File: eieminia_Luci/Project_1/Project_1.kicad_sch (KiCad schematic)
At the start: 10 parts, among them J2 Conn_01x05

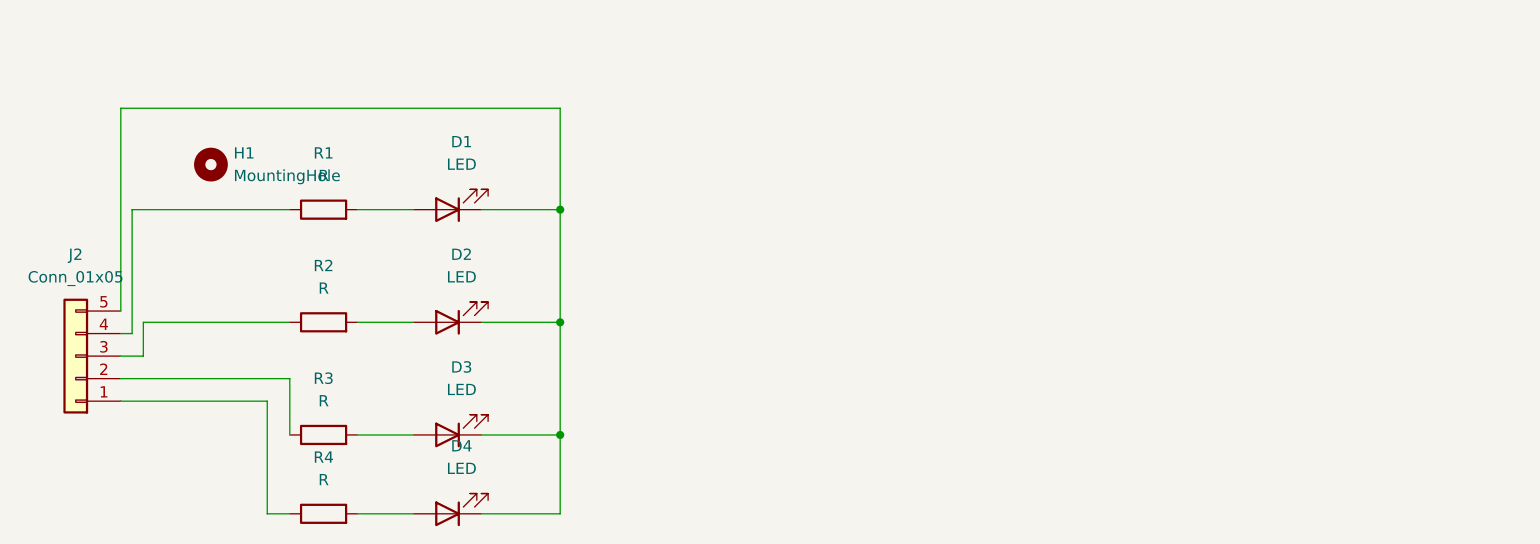
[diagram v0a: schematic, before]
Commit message: Did Stuff
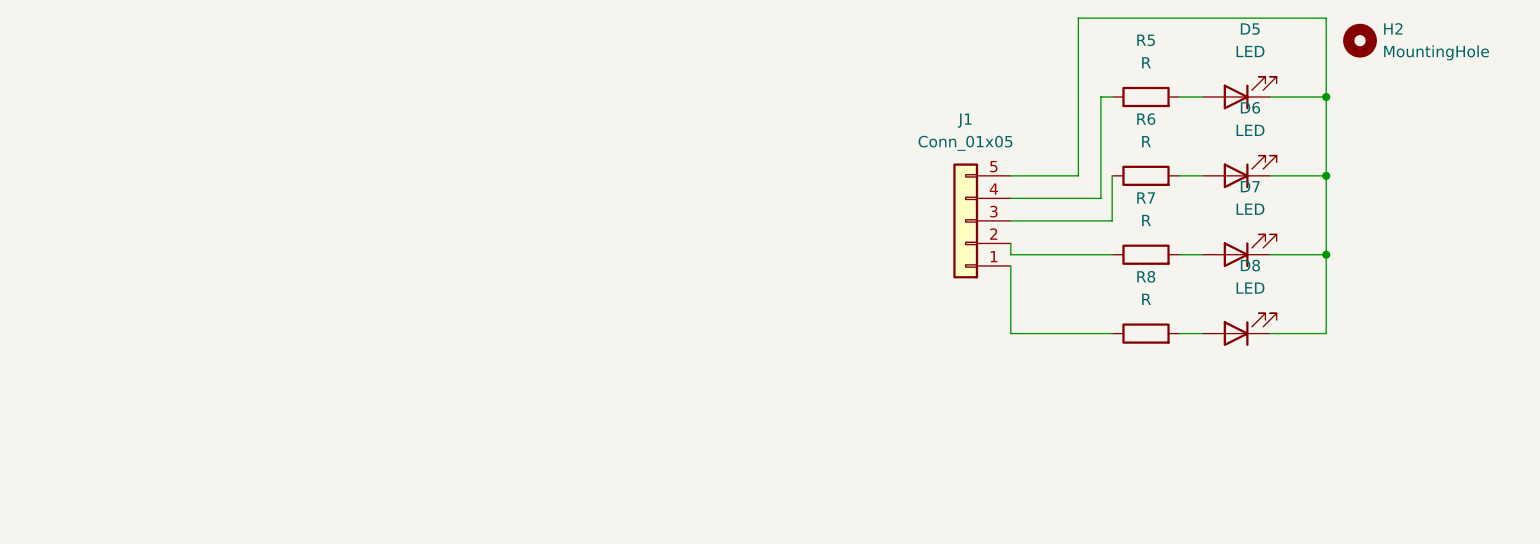
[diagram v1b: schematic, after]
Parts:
- removed D1, D2, D3, D4: LED, LED_THT:LED_D3.0mm, symbol Device:LED
- removed H1: MountingHole, MountingHole:MountingHole_2.2mm_M2, symbol Mechanical:MountingHole
- removed J2: Conn_01x05, Connector_PinHeader_2.54mm:PinHeader_1x05_P2.54mm_Horizontal, symbol Connector_Generic:Conn_01x05
- removed R1, R2, R3, R4: R, Resistor_THT:R_Axial_DIN0411_L9.9mm_D3.6mm_P12.70mm_Horizontal, symbol Device:R
- added D5, D6, D7, D8: LED, LED_THT:LED_D3.0mm, symbol Device:LED
- added H2: MountingHole, MountingHole:MountingHole_2.1mm, symbol Mechanical:MountingHole
- added J1: Conn_01x05, Connector_PinHeader_2.54mm:PinHeader_1x05_P2.54mm_Horizontal, symbol Connector_Generic:Conn_01x05
- added R5, R6, R7, R8: R, Resistor_THT:R_Axial_DIN0309_L9.0mm_D3.2mm_P12.70mm_Horizontal, symbol Device:R
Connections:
- new net: D5.1 (K), D6.1 (K), D7.1 (K), D8.1 (K), J1.5 (Pin_5)
- new net: D8.2 (A), R8.2
- new net: J1.4 (Pin_4), R5.1
- new net: D5.2 (A), R5.2
- new net: J1.3 (Pin_3), R6.1
- new net: D6.2 (A), R6.2
- new net: D7.2 (A), R7.2
- new net: J1.2 (Pin_2), R7.1
- new net: J1.1 (Pin_1), R8.1
